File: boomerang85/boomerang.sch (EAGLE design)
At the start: 16 parts

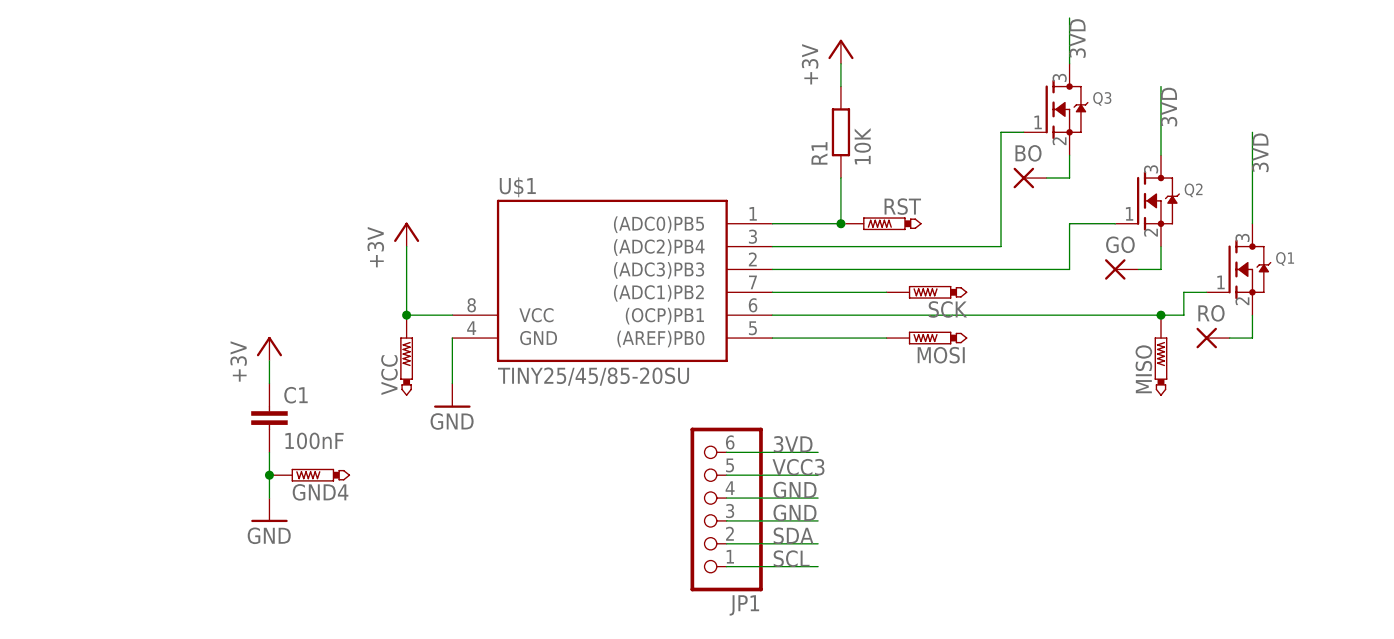
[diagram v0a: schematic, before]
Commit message: moar awesome
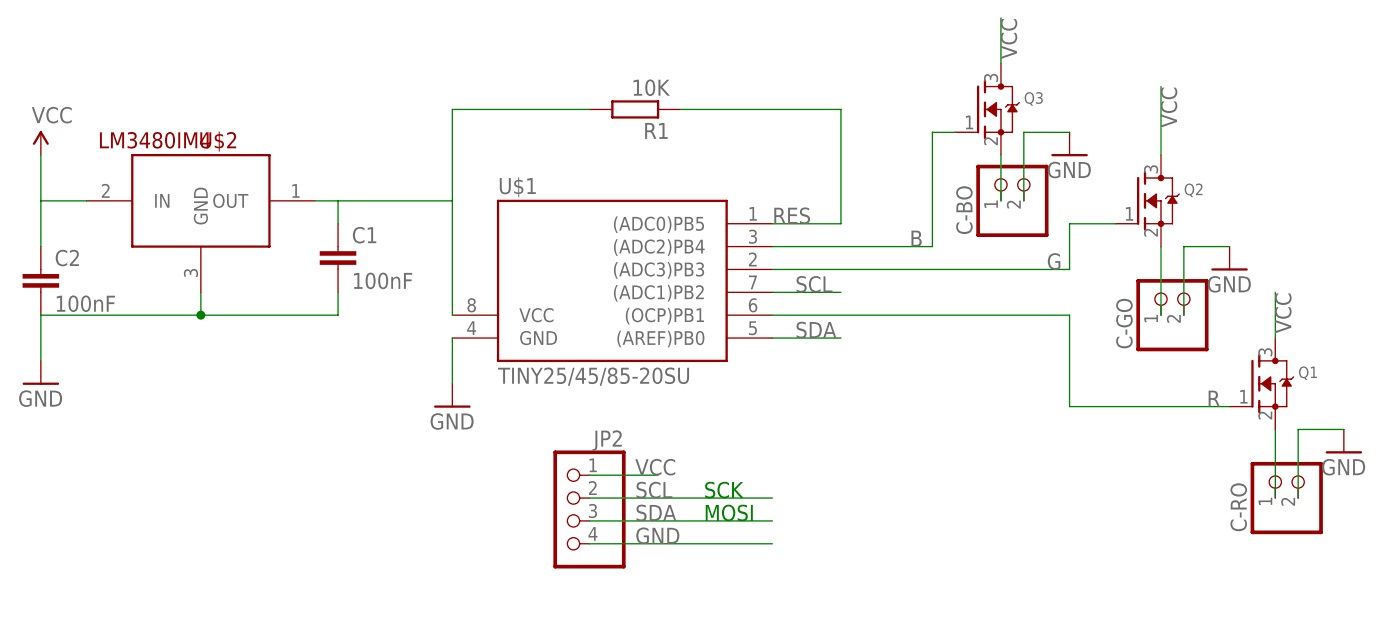
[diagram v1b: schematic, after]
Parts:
- removed BO, GO, RO: (no value), wirepad:SMD2
- removed GND4, MISO, MOSI, RST, SCK, VCC: PTR1TP10R, testpad:PTR1TP10R
- removed JP1: (no value), pinhead:PINHD-1X6/90
- added C-BO, C-GO, C-RO: (no value), pinhead:PINHD-1X2M
- added C2: 100nF, resistor:C-EUC0603
- added JP2: (no value), pinhead-1:PINHD-1X4_2.54-SMD-90°
- added U$2: LM3480IM4, SparkFun-PowerIC:LM3480IM4
- C1: device resistor:C-EUC1206 -> resistor:C-EUC0603
- R1: device resistor:R-EU_R1206 -> resistor:R-EU_R0603
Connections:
- removed net 3VD: JP1.6, Q1.D, Q2.D, Q3.D
- removed net VCC3: C1.1, JP1.5, R1.2, U$1.VCC, VCC.TP
- new net VCC: C2.1, JP2.1, Q1.D, Q2.D, Q3.D, U$2.IN
- new net VCC_GOOD: C1.1, R1.2, U$1.VCC, U$2.OUT
- net BO: now also C-BO.1; no longer BO.P
- net GND: now also C-BO.2, C-GO.2, C-RO.2, C2.2, JP2.4, U$2.GND; no longer GND4.TP, JP1.3, JP1.4
- net GO: now also C-GO.1; no longer GO.P
- net R: no longer MISO.TP
- net RES: no longer RST.TP
- net RO: now also C-RO.1; no longer RO.P
- net SCL: now also JP2.2; no longer JP1.1, SCK.TP
- net SDA: now also JP2.3; no longer JP1.2, MOSI.TP
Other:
- note added: "MOSI"
- note added: "SCK"
- moved on the sheet: C1, Q1, Q3, R1
